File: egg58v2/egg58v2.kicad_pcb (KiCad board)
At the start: 2 copper layers, 141.1 x 125.8 mm, 37 parts, among them J1 AudioJack4, SW11 SW_PUSH_LED, SW12 SW_PUSH_LED, SW13 SW_PUSH_LED, SW14 SW_PUSH_LED, SW15 SW_PUSH_LED, SW16 SW_PUSH_LED, SW21 SW_PUSH_LED, SW22 SW_PUSH_LED, SW23 SW_PUSH_LED, SW24 SW_PUSH_LED, SW25 SW_PUSH_LED, SW26 SW_PUSH_LED, SW31 SW_PUSH_LED, SW32 SW_PUSH_LED, SW33 SW_PUSH_LED, SW34 SW_PUSH_LED, SW35 SW_PUSH_LED, SW36 SW_PUSH_LED, SW41 SW_PUSH_LED, SW42 SW_PUSH_LED, SW43 SW_PUSH_LED, SW44 SW_PUSH_LED, SW45 SW_PUSH_LED, SW46 SW_PUSH_LED, SW52 SW_PUSH_LED, SW53 SW_PUSH_LED, SW54 SW_PUSH_LED, SW55 SW_PUSH_LED, SW56 SW_PUSH_LED, U1 Elite-C

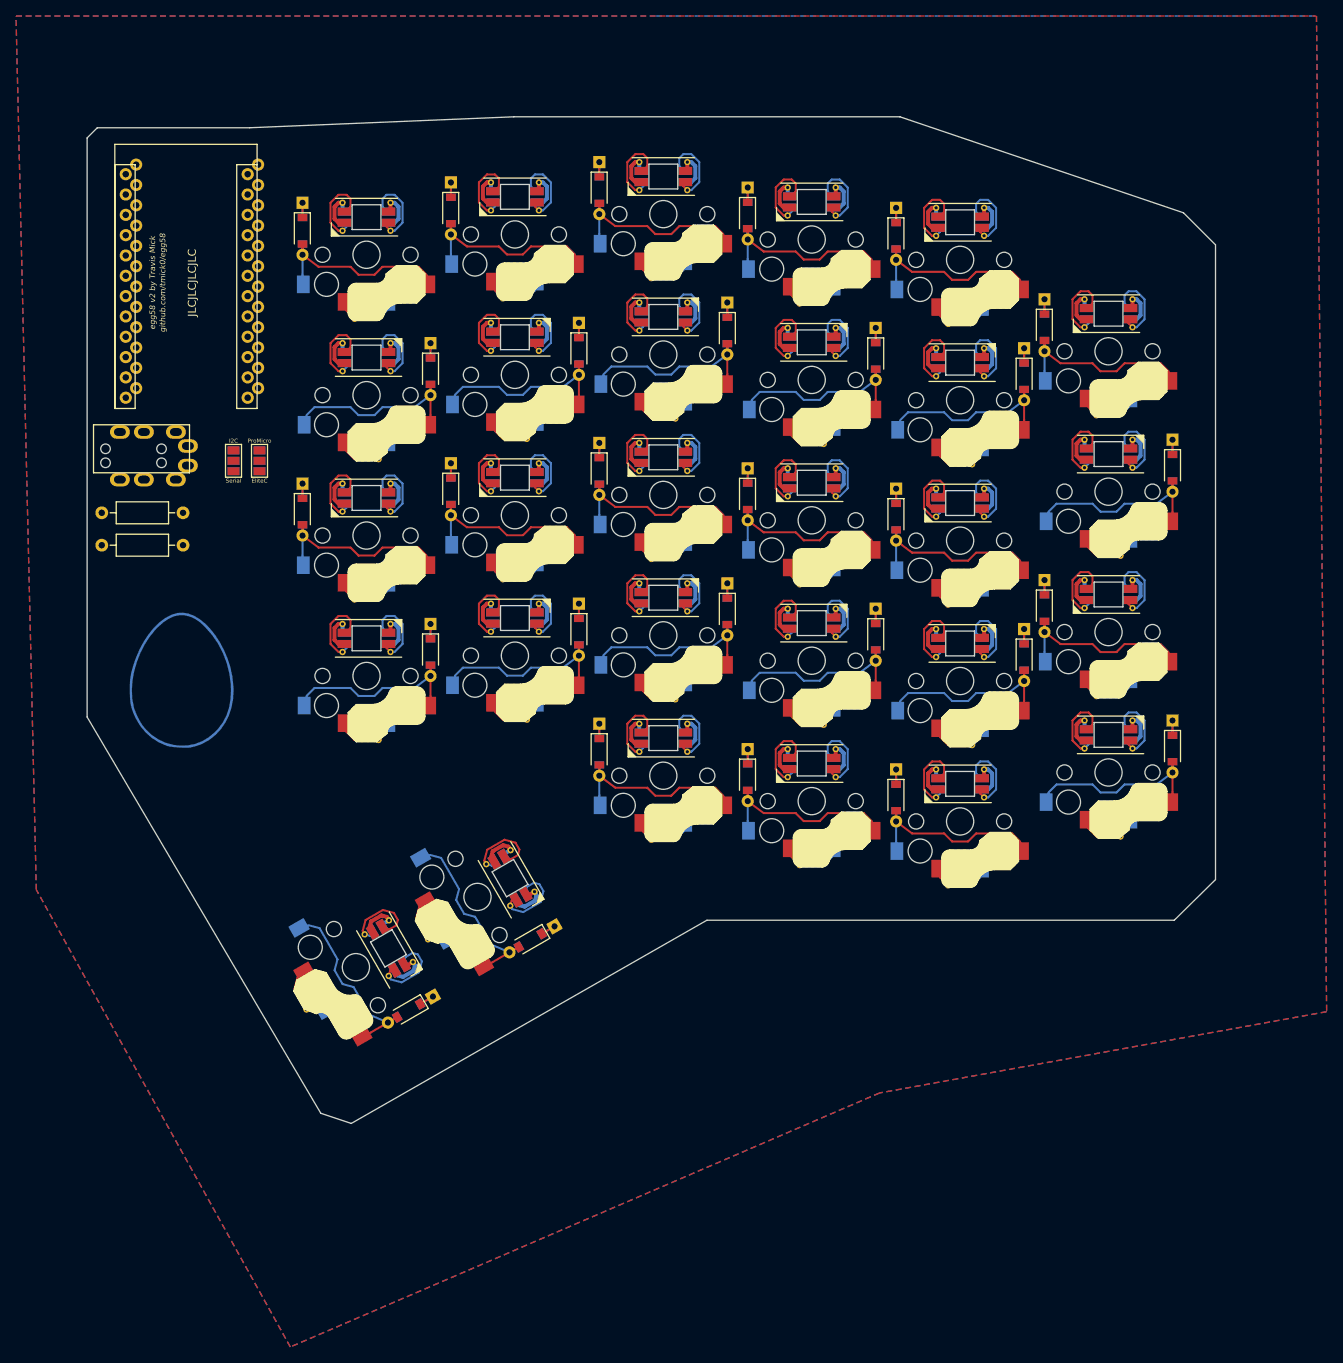
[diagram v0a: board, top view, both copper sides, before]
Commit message: starting routing
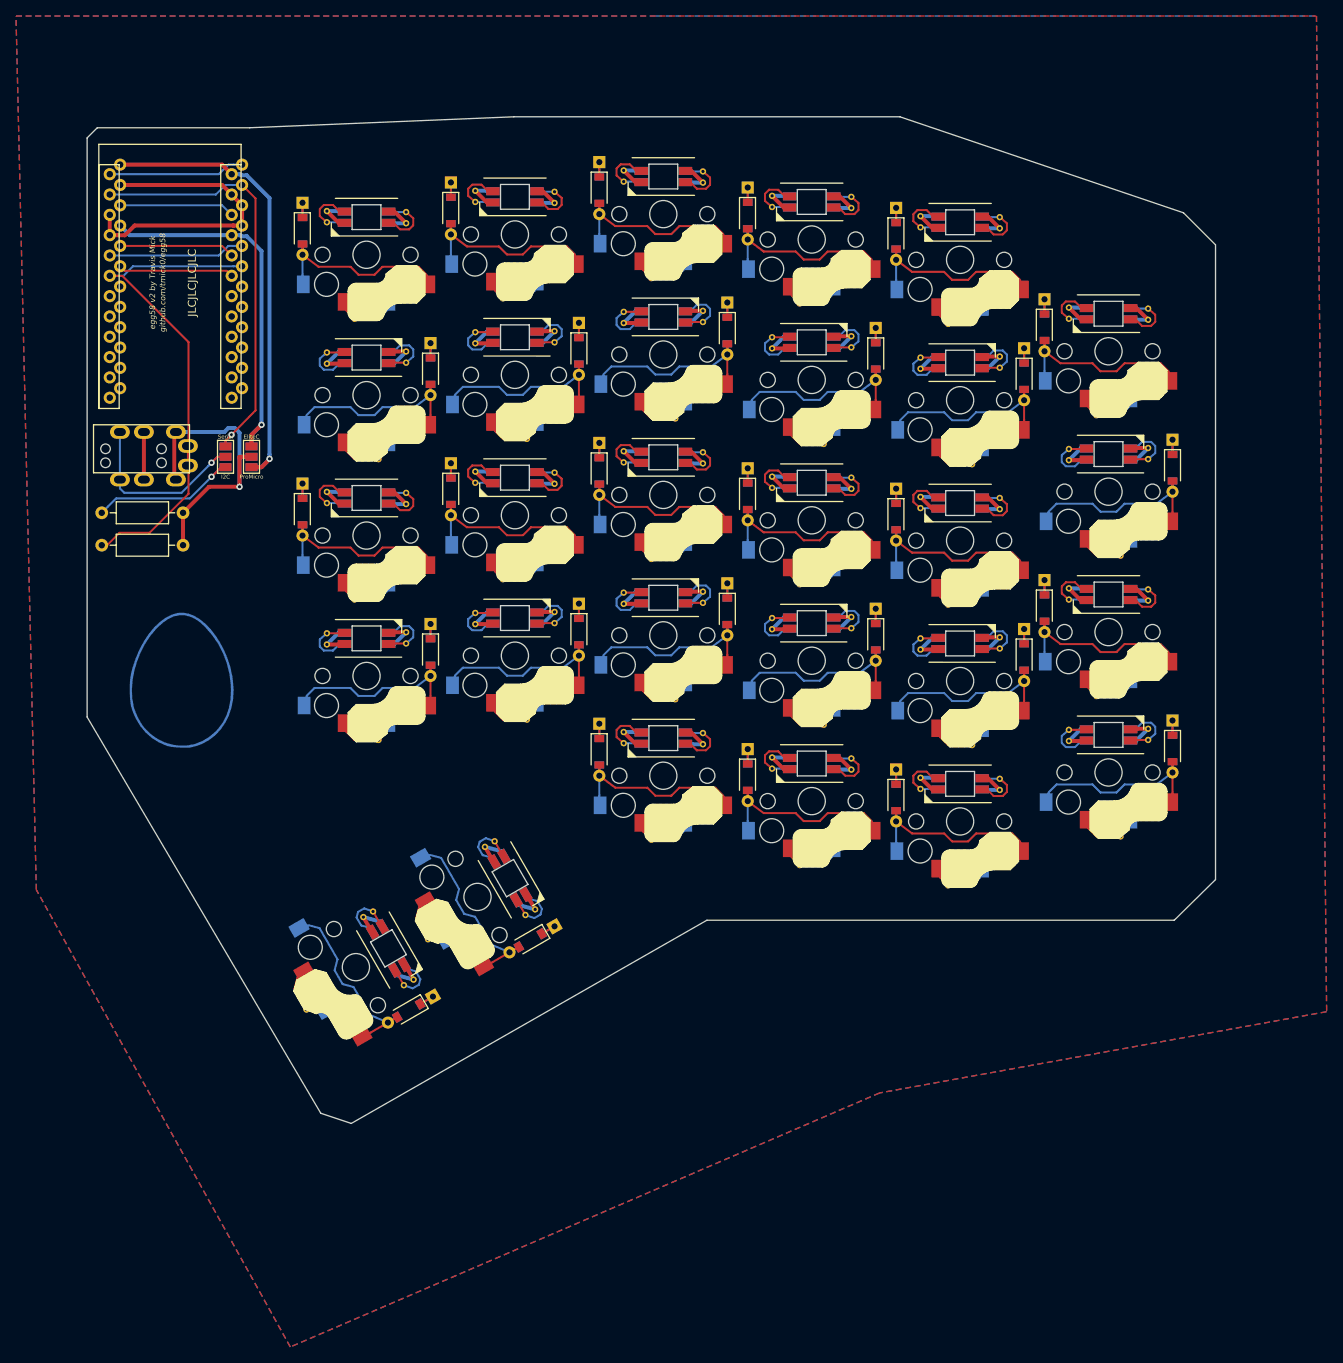
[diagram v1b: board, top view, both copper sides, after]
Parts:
- moved U1 2.00 mm to (118.5, 58.8)
- moved JP1 1.12 mm to (128.5, 80.5), turned to 90 degrees
- moved JP2 1.12 mm to (125.2, 80.5), turned to 270 degrees
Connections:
- SW11 pad 1: VDD -> VCC
- SW12 pad 1: VDD -> VCC
- SW13 pad 1: VDD -> VCC
- SW14 pad 1: VDD -> VCC
- SW15 pad 1: VDD -> VCC
- SW16 pad 1: VDD -> VCC
- SW21 pad 1: VDD -> VCC
- SW22 pad 1: VDD -> VCC
- SW23 pad 1: VDD -> VCC
- SW24 pad 1: VDD -> VCC
- SW25 pad 1: VDD -> VCC
- SW26 pad 1: VDD -> VCC
- SW31 pad 1: VDD -> VCC
- SW32 pad 1: VDD -> VCC
- SW33 pad 1: VDD -> VCC
- SW34 pad 1: VDD -> VCC
- SW35 pad 1: VDD -> VCC
- SW36 pad 1: VDD -> VCC
- SW41 pad 1: VDD -> VCC
- SW42 pad 1: VDD -> VCC
- SW43 pad 1: VDD -> VCC
- SW44 pad 1: VDD -> VCC
- SW45 pad 1: VDD -> VCC
- SW46 pad 1: VDD -> VCC
- SW52 pad 1: VDD -> VCC
- SW53 pad 1: VDD -> VCC
- SW54 pad 1: VDD -> VCC
- SW55 pad 1: VDD -> VCC
- SW56 pad 1: VDD -> VCC
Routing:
- net SCL: track 0.00 -> 62.8 mm
- net VBUS: track 0.00 -> 58.4 mm, vias 0 -> 1
- net SERIAL: track 0.00 -> 53.7 mm, vias 0 -> 1
- net VREG: track 0.00 -> 47.1 mm, vias 0 -> 1
- net GND: track 0.00 -> 44.4 mm
- net VCC: track 0.00 -> 40.6 mm, vias 0 -> 1
- net SDA: track 0.00 -> 37.1 mm, vias 0 -> 1
- net DATA: track 0.00 -> 24.4 mm, vias 0 -> 1
- net RGB: track 0.00 -> 17.0 mm
- net Net-(U1-Pad20): track 0.00 -> 14.4 mm
- net Net-(U1-Pad22): track 0.00 -> 14.4 mm
- net Net-(U1-Pad19): track 0.00 -> 14.4 mm
